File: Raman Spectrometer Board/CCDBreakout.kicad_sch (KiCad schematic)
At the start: 1 part

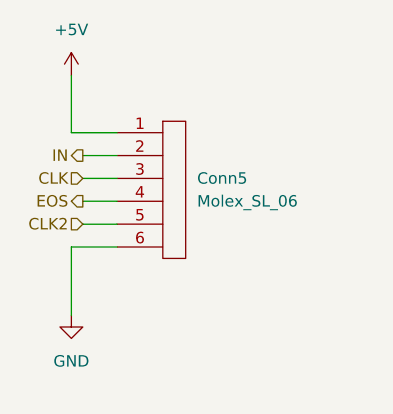
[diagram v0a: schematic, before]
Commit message: ST and EOS Pin Connections
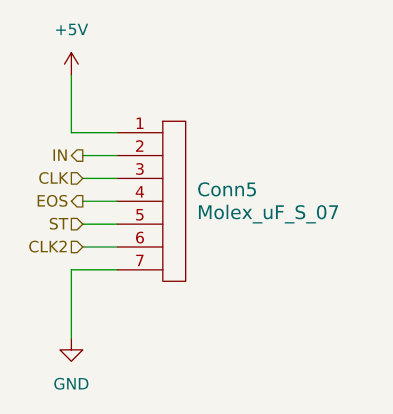
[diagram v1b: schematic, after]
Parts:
- removed Conn5: Molex_SL_06, symbol MRDT_Connectors:Molex_SL_06
- added Conn5: Molex_uF_S_07, MRDT_Connectors:MOLEX_uF_S_07_Horizontal, symbol MRDT_Connectors:Molex_uF_S_07
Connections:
- net +5V: now also Conn5.1
- net CLK: now also Conn5.3
- net CLK2: now also Conn5.6
- net EOS: now also Conn5.4
- net GND: now also Conn5.7
- net IN: now also Conn5.2
- new net ST: Conn5.5
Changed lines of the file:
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@@
+	(wire
+		(pts
+			(xy 154.94 102.87) (xy 158.75 102.87)
+		)
+		(stroke
+			(width 0)
+			(type default)
+		)
+	)
 	(wire
 		(pts
@@
 	(wire
 		(pts
-			(xy 153.67 113.03) (xy 153.67 105.41)
-		)
-		(stroke
-			(width 0)
-			(type default)
-		)
-	)
-	(wire
-		(pts
-			(xy 153.67 105.41) (xy 158.75 105.41)
+			(xy 153.67 115.57) (xy 153.67 107.95)
 		)
 		(stroke
@@
 	(wire
 		(pts
+			(xy 154.94 105.41) (xy 158.75 105.41)
+		)
+		(stroke
+			(width 0)
+			(type default)
+		)
+	)
+	(wire
+		(pts
 			(xy 154.94 100.33) (xy 158.75 100.33)
 		)
@@
 	(wire
 		(pts
-			(xy 154.94 102.87) (xy 158.75 102.87)
+			(xy 153.67 107.95) (xy 158.75 107.95)
 		)
 		(stroke
@@
 	(hierarchical_label "CLK2"
 		(shape input)
-		(at 154.94 102.87 180)
+		(at 154.94 105.41 180)
 		(effects
 			(font
@@
 		)
 	)
+	(hierarchical_label "ST"
+		(shape input)
+		(at 154.94 102.87 180)
+		(effects
+			(font
+				(size 1.27 1.27)
+			)
+			(justify right)
+		)
+	)
 	(symbol
-		(lib_id "MRDT_Connectors:Molex_SL_06")
-		(at 163.83 106.68 0)
+		(lib_id "MRDT_Connectors:Molex_uF_S_07")
+		(at 163.83 109.22 0)
 		(unit 1)
 		(exclude_from_sim no)
@@
 		(fields_autoplaced yes)
 		(property "Reference" "Conn5"
-			(at 167.64 97.7899 0)
-			(effects
-				(font
-					(size 1.27 1.27)
+			(at 167.64 99.0599 0)
+			(effects
+				(font
+					(size 1.524 1.524)
 				)
 				(justify left)
 			)
 		)
-		(property "Value" "Molex_SL_06"
-			(at 167.64 100.3299 0)
-			(effects
-				(font
-					(size 1.27 1.27)
+		(property "Value" "Molex_uF_S_07"
+			(at 167.64 101.5999 0)
+			(effects
+				(font
+					(size 1.524 1.524)
 				)
 				(justify left)
 			)
 		)
-		(property "Footprint" ""
-			(at 158.75 102.87 0)
-			(effects
-				(font
-					(size 1.27 1.27)
+		(property "Footprint" "MRDT_Connectors:MOLEX_uF_S_07_Horizontal"
+			(at 163.83 104.14 0)
+			(effects
+				(font
+					(size 1.524 1.524)
 				)
 				(hide yes)
@@
 		)
 		(property "Datasheet" ""
-			(at 158.75 102.87 0)
-			(effects
-				(font
-					(size 1.27 1.27)
+			(at 163.83 104.14 0)
+			(effects
+				(font
+					(size 1.524 1.524)
 				)
 				(hide yes)
@@
 		)
 		(property "Description" ""
-			(at 158.75 102.87 0)
+			(at 163.83 109.22 0)
 			(effects
 				(font
@@
 		(pin "5"
 		)
+		(pin "2"
+		)
+		(pin "4"
+		)
+		(pin "7"
+		)
+		(pin "1"
+		)
+		(pin "6"
+		)
 		(pin "3"
-		)
-		(pin "2"
-		)
-		(pin "1"
-		)
-		(pin "6"
-		)
-		(pin "4"
 		)
 		(instances
@@
 	(symbol
 		(lib_id "power:GND")
-		(at 153.67 113.03 0)
+		(at 153.67 115.57 0)
 		(unit 1)
 		(exclude_from_sim no)
@@
 		(fields_autoplaced yes)
 		(property "Reference" "#PWR027"
-			(at 153.67 119.38 0)
+			(at 153.67 121.92 0)
 			(effects
 				(font
@@
 		)
 		(property "Value" "GND"
-			(at 153.67 118.11 0)
+			(at 153.67 120.65 0)
 			(effects
 				(font
@@
 		)
 		(property "Footprint" ""
-			(at 153.67 113.03 0)
+			(at 153.67 115.57 0)
 			(effects
 				(font
@@
 		)
 		(property "Datasheet" ""
-			(at 153.67 113.03 0)
+			(at 153.67 115.57 0)
 			(effects
 				(font
@@
 		)
 		(property "Description" "Power symbol creates a global label with name \"GND\" , ground"
-			(at 153.67 113.03 0)
-			(effects
-				(font
+			(at 153.67 115.57 0)
+			(effects
+				(font
